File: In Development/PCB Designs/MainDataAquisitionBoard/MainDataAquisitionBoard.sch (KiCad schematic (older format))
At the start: 22 parts, among them J4 1x24, J5 Teensy 3.6L, J6 Teensy 3.6R, J7 1x24

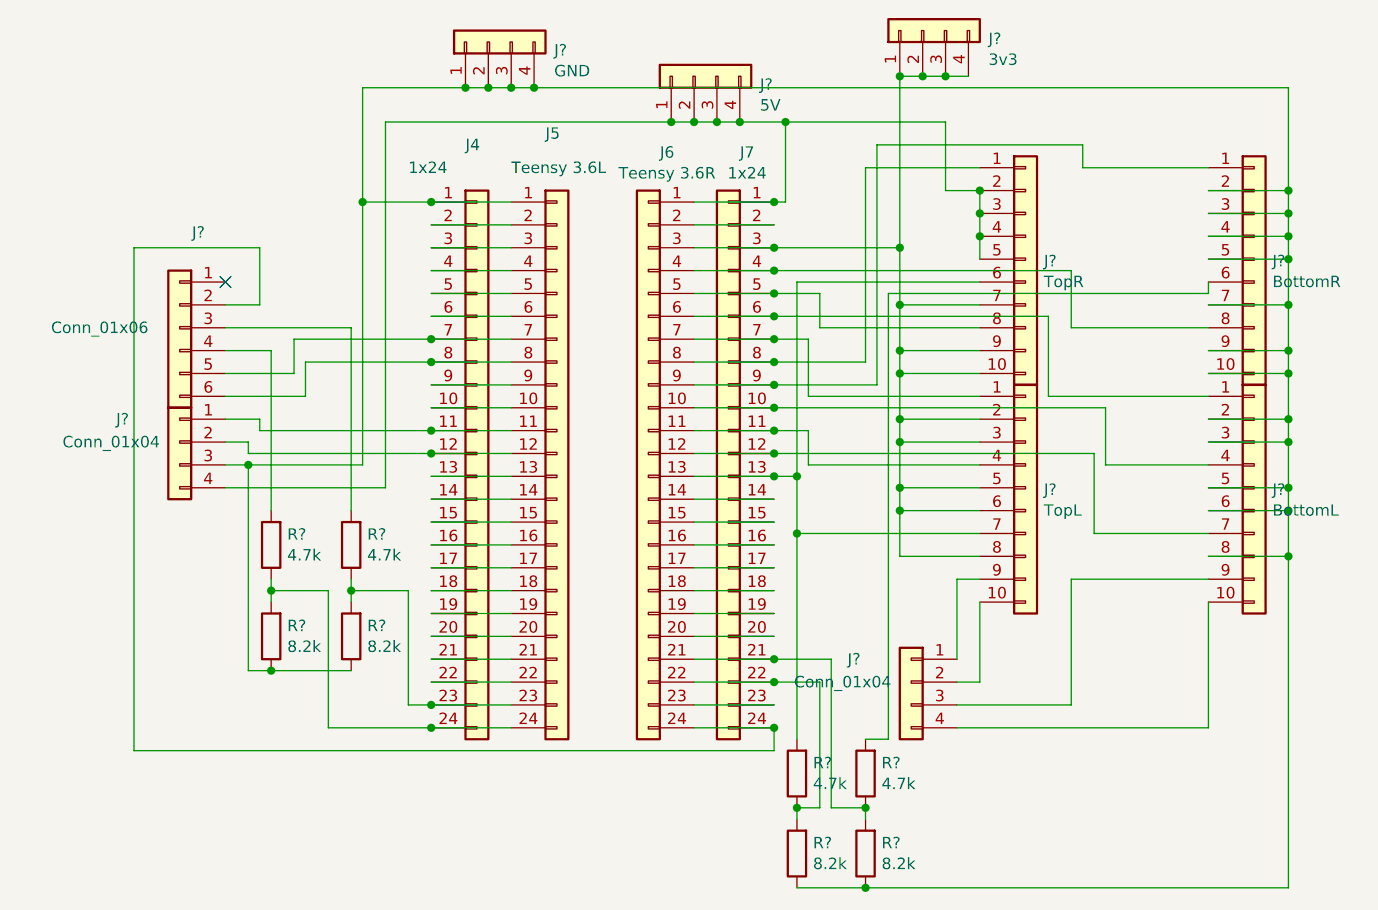
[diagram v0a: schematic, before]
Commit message: Finished main DAQ PCB
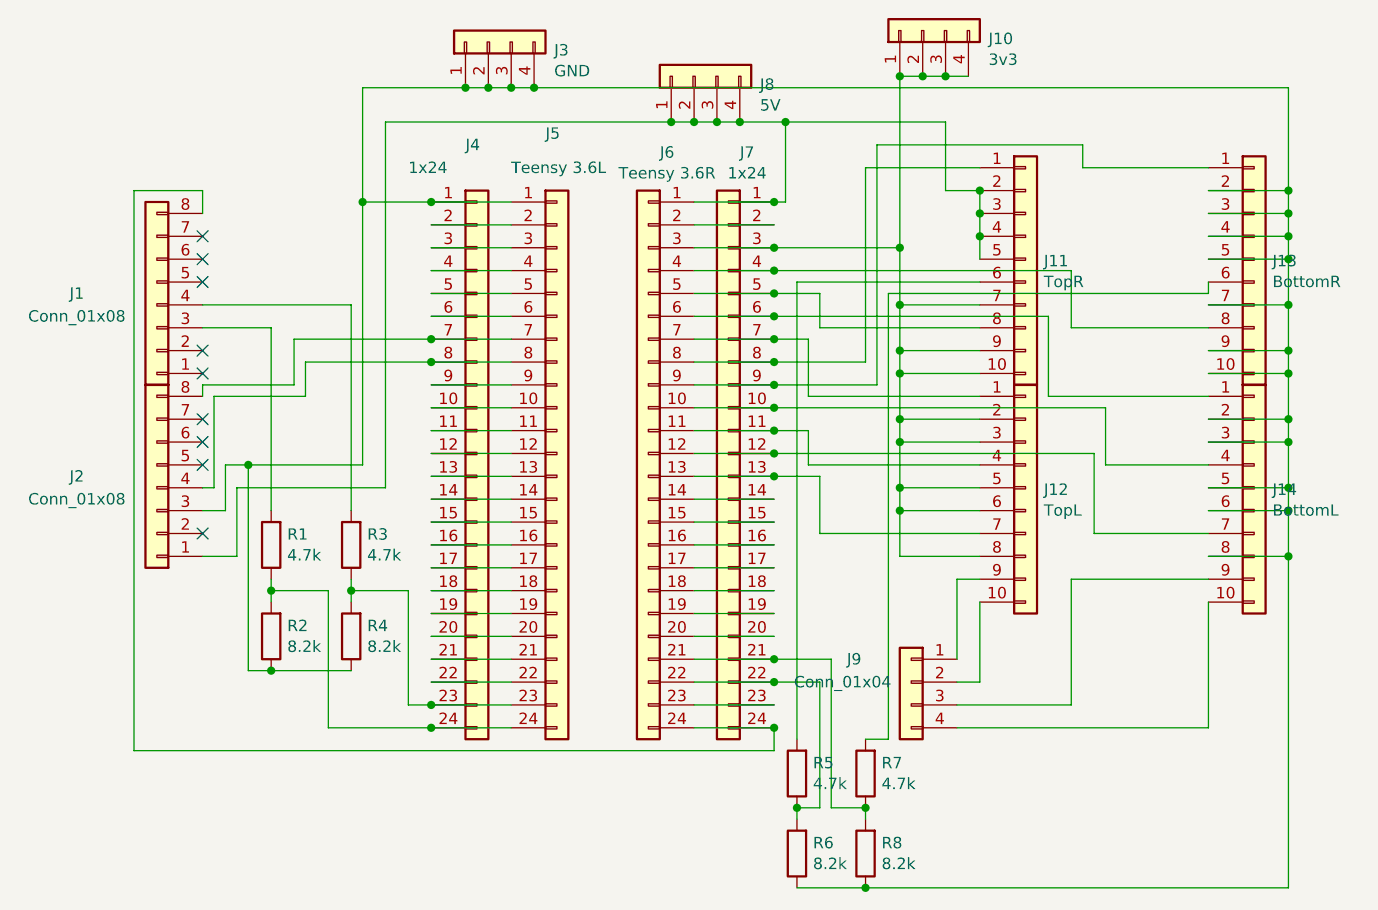
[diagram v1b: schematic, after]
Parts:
- removed J?: Conn_01x06, symbol Connector_Generic:Conn_01x06
- removed J?: Conn_01x04, symbol Connector_Generic:Conn_01x04
- added J1, J2: Conn_01x08, Connector_PinHeader_2.00mm:PinHeader_1x08_P2.00mm_Vertical, symbol Connector_Generic:Conn_01x08
- J10, J3, J8, J9: renamed from J?; footprint (none) -> Connector_PinHeader_2.54mm:PinHeader_1x04_P2.54mm_Vertical
- J11, J12, J13, J14: renamed from J?; footprint (none) -> CustomKiCADLibrary:PinHeader_1x10_P5.08mm_Vertical
- R1, R2, R3, R4, R5, R6, R7, R8: renamed from R?; footprint (none) -> Resistor_THT:R_Axial_DIN0207_L6.3mm_D2.5mm_P7.62mm_Horizontal
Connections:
- net at J13.10 (Pin_10), J13.2 (Pin_2), J13.3 (Pin_3)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: now also J2.3 (Pin_3)
- net at J4.7 (Pin_7), J5.7 (Pin_7): now also J2.8 (Pin_8)
- net at J4.8 (Pin_8), J5.8 (Pin_8): now also J2.4 (Pin_4)
- net at J11.2 (Pin_2), J11.3 (Pin_3), J11.4 (Pin_4)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: now also J2.1 (Pin_1)
- net at J12.7 (Pin_7), J6.13 (Pin_13), J7.13 (Pin_13): no longer J11.6 (Pin_6), R5.2
- net at J6.24 (Pin_24), J7.24 (Pin_24): now also J1.8 (Pin_8)
- net at R3.2: now also J1.4 (Pin_4)
- net at R1.2: now also J1.3 (Pin_3)
- new net: J11.6 (Pin_6), R5.2
- no-connect marks 1 -> 9
